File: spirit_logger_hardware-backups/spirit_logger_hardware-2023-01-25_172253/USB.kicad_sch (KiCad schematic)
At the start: 22 parts, among them J3 USB_C_Receptacle, U4 SN74LVC1G00DRY2, U5 74CBTLV3245BQ

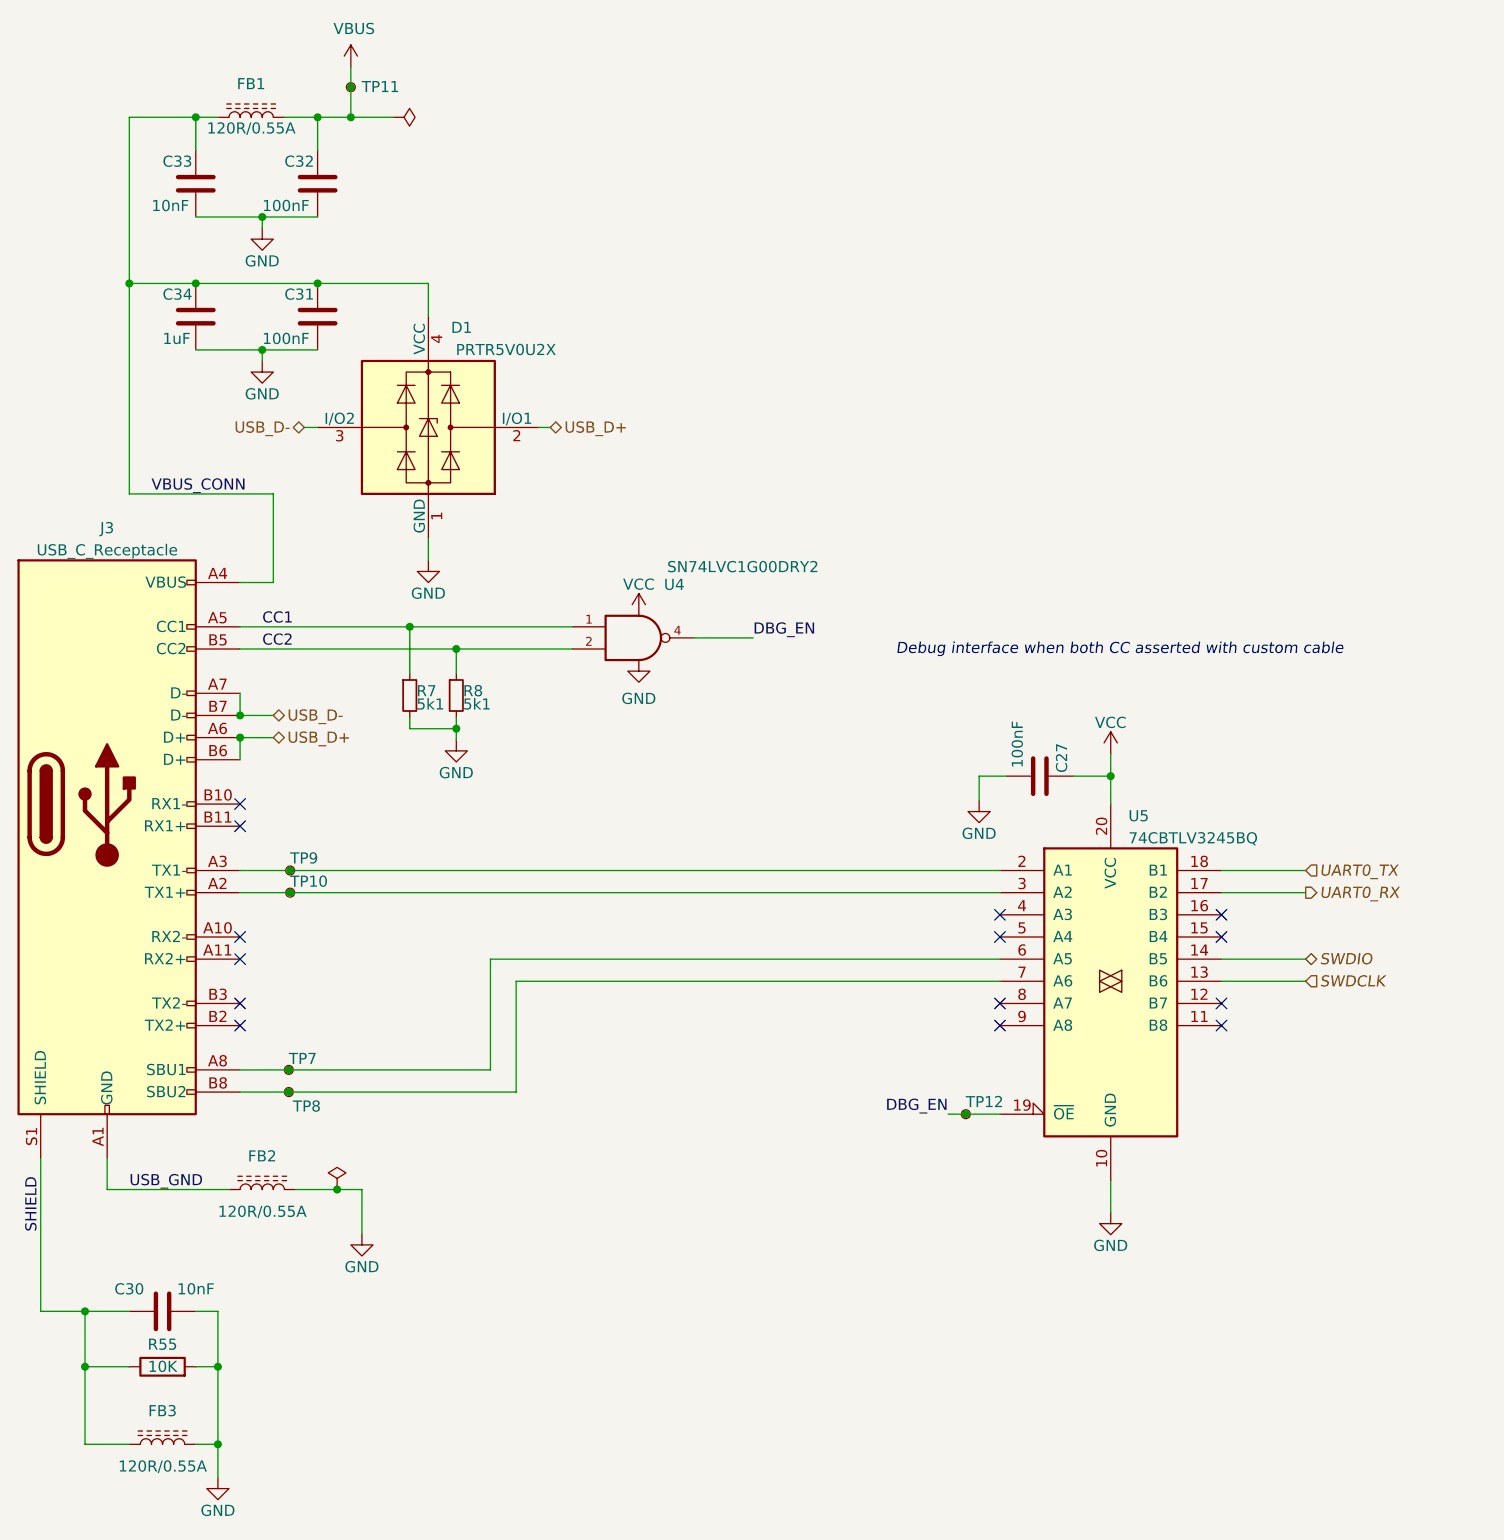
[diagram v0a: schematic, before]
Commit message: drc and packaging
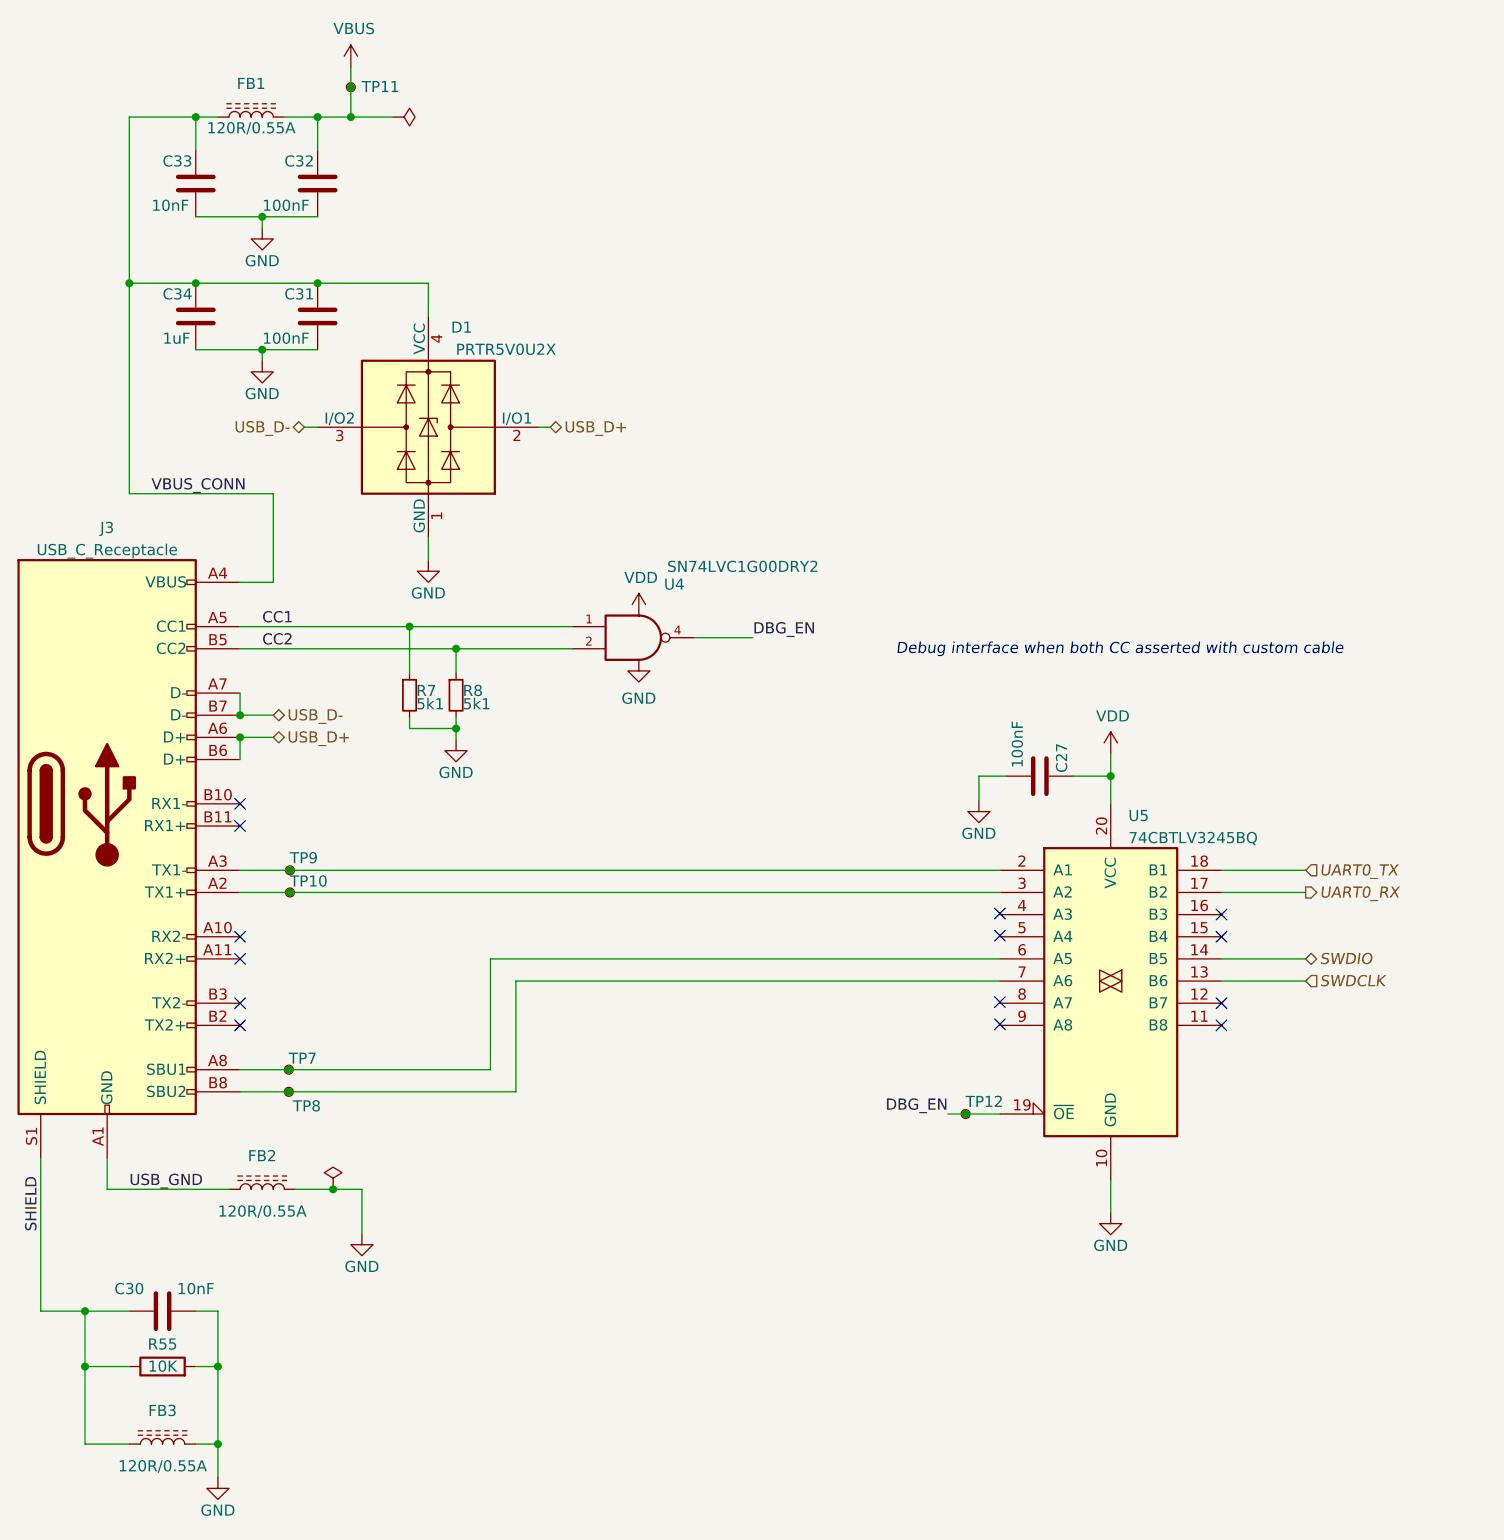
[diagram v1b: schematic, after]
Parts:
- J3: footprint Connector_USB:USB_C_Receptacle_GCT_USB4105-xx-A_16P_TopMnt_Horizontal -> Connector_USB.pretty:USB_C_Receptacle_GCT_USB4105-xx-A_16P_TopMnt_Horizontal
- R55: footprint Resistor_SMD:R_0201_0603Metric -> MCU_Nordic_Accessory:R_0201
- R7, R8: footprint Resistor_SMD:R_0201_0603Metric -> Resistor_SMD.pretty:R_0402_1005Metric
- TP10, TP11, TP12, TP7, TP8, TP9: footprint tuna-f1sh/jbr-kicad/Misc.pretty:TestPoint_Pad_D1.0mm_Tight -> tunaf1sh/misc.pretty:TestPoint_Pad_D1.0mm_Tight
- U5: footprint tuna-f1sh/jbr-kicad/SnapEDA.pretty:QFN50P450X250X100-21N -> tunaf1sh/snapeda.pretty:QFN50P450X250X100-21N
